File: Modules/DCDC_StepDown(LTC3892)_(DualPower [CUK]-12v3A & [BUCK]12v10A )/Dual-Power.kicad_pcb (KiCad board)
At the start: 4 copper layers, 58.4 x 55.9 mm, 81 parts, among them J1 Conn_02x05_Top_Bottom, J2 Conn_02x05_Top_Bottom, J3 Conn_01x02, Q1 BSC028N06LS3, Q2 BSC028N06LS3, Q3 BSC028N06LS3, Q4 BSC028N06LS3, Q5 BSC028N06LS3, U1 LTC3892EUHPBF, U2 LT1797

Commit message: update Dual-power
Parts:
- C11: value 1nF -> 6.8nF
- C12: value 100pF -> 47pF
- C21, C25: value 1nF -> 220pF
- C5: value 10nF -> 6.8nF
- C6: value 330pF -> 47pF
- R3: value 7.5K -> 10K
- R4: value 34.8K -> 10K
- R5: value 100K -> 31.6K

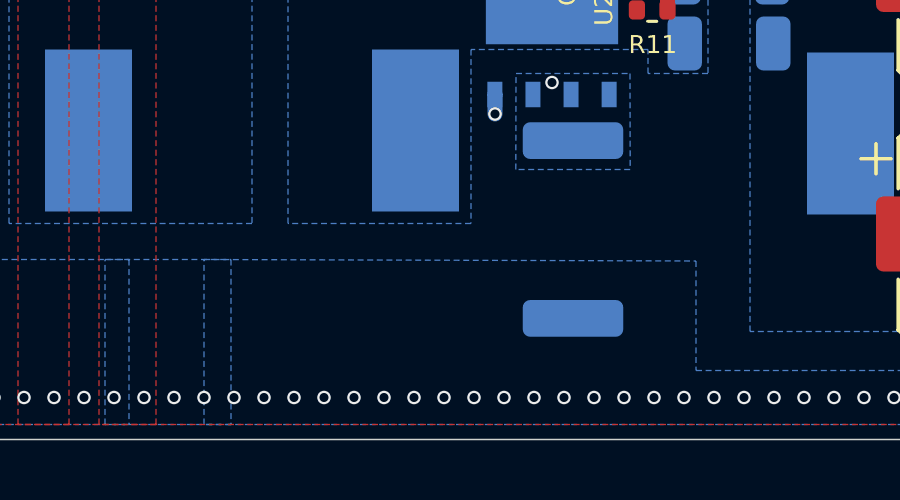
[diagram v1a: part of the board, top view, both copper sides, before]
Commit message: update dual_power
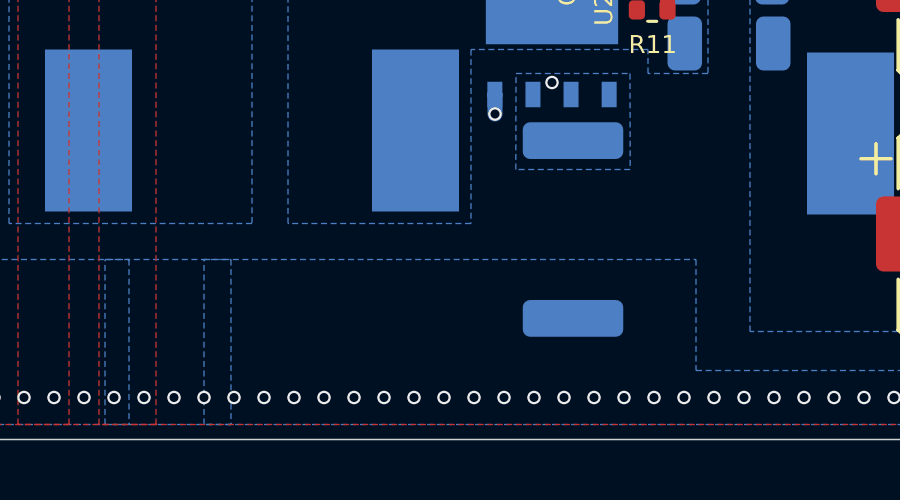
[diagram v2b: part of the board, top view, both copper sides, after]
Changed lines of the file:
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@@
     )
     (fp_poly (pts
+        (xy -1.675 0.1)
+        (xy -1.675 1.675)
+        (xy -0.1 1.675)
+        (xy -0.1 0.1)
+      ) (layer "F.Paste") (width 0.0254) (fill solid))
+    (fp_poly (pts
         (xy 0.1 0.1)
         (xy 0.1 1.675)
@@
         (xy -0.1 -1.675)
       ) (layer "F.Paste") (width 0.0254) (fill solid))
-    (fp_poly (pts
-        (xy -1.675 0.1)
-        (xy -1.675 1.675)
-        (xy -0.1 1.675)
-        (xy -0.1 0.1)
-      ) (layer "F.Paste") (width 0.0254) (fill solid))
-    (fp_line (start 2.667 -2.2352) (end 2.667 -2.667) (layer "F.SilkS") (width 0.1524))
     (fp_line (start -2.2352 -2.667) (end -2.667 -2.667) (layer "F.SilkS") (width 0.1524))
+    (fp_line (start 2.667 2.667) (end 2.667 2.2352) (layer "F.SilkS") (width 0.1524))
     (fp_line (start -2.667 -2.667) (end -2.667 -2.2352) (layer "F.SilkS") (width 0.1524))
+    (fp_line (start 2.667 -2.667) (end 2.2352 -2.667) (layer "F.SilkS") (width 0.1524))
+    (fp_line (start 2.2352 2.667) (end 2.667 2.667) (layer "F.SilkS") (width 0.1524))
+    (fp_line (start 2.667 -2.2352) (end 2.667 -2.667) (layer "F.SilkS") (width 0.1524))
     (fp_line (start -2.667 2.2352) (end -2.667 2.667) (layer "F.SilkS") (width 0.1524))
     (fp_line (start -2.667 2.667) (end -2.2352 2.667) (layer "F.SilkS") (width 0.1524))
-    (fp_line (start 2.2352 2.667) (end 2.667 2.667) (layer "F.SilkS") (width 0.1524))
-    (fp_line (start 2.667 -2.667) (end 2.2352 -2.667) (layer "F.SilkS") (width 0.1524))
-    (fp_line (start 2.667 2.667) (end 2.667 2.2352) (layer "F.SilkS") (width 0.1524))
-    (fp_line (start 0.889 -2.54) (end 0.6096 -2.54) (layer "F.Fab") (width 0.1524))
-    (fp_line (start -0.4064 2.54) (end -0.1016 2.54) (layer "F.Fab") (width 0.1524))
-    (fp_line (start 1.0922 2.54) (end 1.397 2.54) (layer "F.Fab") (width 0.1524))
-    (fp_line (start 0.4064 -2.54) (end 0.1016 -2.54) (layer "F.Fab") (width 0.1524))
-    (fp_line (start -1.6002 -2.54) (end -1.905 -2.54) (layer "F.Fab") (width 0.1524))
-    (fp_line (start 2.54 0.889) (end 2.54 0.6096) (layer "F.Fab") (width 0.1524))
-    (fp_line (start 2.54 -0.1016) (end 2.54 -0.4064) (layer "F.Fab") (width 0.1524))
     (fp_line (start 2.54 -0.6096) (end 2.54 -0.889) (layer "F.Fab") (width 0.1524))
-    (fp_line (start -2.54 -1.27) (end -1.27 -2.54) (layer "F.Fab") (width 0.1524))
-    (fp_line (start -2.54 2.54) (end 2.54 2.54) (layer "F.Fab") (width 0.1524))
-    (fp_line (start -2.54 -0.889) (end -2.54 -0.6096) (layer "F.Fab") (width 0.1524))
-    (fp_line (start -1.905 2.54) (end -1.6002 2.54) (layer "F.Fab") (width 0.1524))
+    (fp_line (start -0.1016 -2.54) (end -0.4064 -2.54) (layer "F.Fab") (width 0.1524))
+    (fp_line (start 0.4064 -2.54) (end 0.1016 -2.54) (layer "F.Fab") (width 0.1524))
     (fp_line (start -0.6096 -2.54) (end -0.889 -2.54) (layer "F.Fab") (width 0.1524))
+    (fp_line (start -2.54 -1.27) (end -1.27 -2.54) (layer "F.Fab") (width 0.1524))
+    (fp_line (start 2.54 -2.54) (end -2.54 -2.54) (layer "F.Fab") (width 0.1524))
     (fp_line (start 2.54 0.4064) (end 2.54 0.1016) (layer "F.Fab") (width 0.1524))
-    (fp_line (start 2.54 1.905) (end 2.54 1.6002) (layer "F.Fab") (width 0.1524))
-    (fp_line (start -2.54 -0.4064) (end -2.54 -0.1016) (layer "F.Fab") (width 0.1524))
     (fp_line (start -2.54 -2.54) (end -2.54 2.54) (layer "F.Fab") (width 0.1524))
-    (fp_line (start 2.54 -1.0922) (end 2.54 -1.397) (layer "F.Fab") (width 0.1524))
-    (fp_line (start -0.1016 -2.54) (end -0.4064 -2.54) (layer "F.Fab") (width 0.1524))
-    (fp_line (start 2.54 -2.54) (end -2.54 -2.54) (layer "F.Fab") (width 0.1524))
-    (fp_line (start -0.889 2.54) (end -0.6096 2.54) (layer "F.Fab") (width 0.1524))
+    (fp_line (start 0.1016 2.54) (end 0.4064 2.54) (layer "F.Fab") (width 0.1524))
+    (fp_line (start 2.54 1.397) (end 2.54 1.0922) (layer "F.Fab") (width 0.1524))
     (fp_line (start -2.54 1.0922) (end -2.54 1.397) (layer "F.Fab") (width 0.1524))
+    (fp_line (start -1.905 2.54) (end -1.6002 2.54) (layer "F.Fab") (width 0.1524))
+    (fp_line (start -2.54 -0.889) (end -2.54 -0.6096) (layer "F.Fab") (width 0.1524))
+    (fp_line (start 1.397 -2.54) (end 1.0922 -2.54) (layer "F.Fab") (width 0.1524))
+    (fp_line (start -2.54 -0.4064) (end -2.54 -0.1016) (layer "F.Fab") (width 0.1524))
+    (fp_line (start 2.54 2.54) (end 2.54 -2.54) (layer "F.Fab") (width 0.1524))
     (fp_line (start 2.54 -1.6002) (end 2.54 -1.905) (layer "F.Fab") (width 0.1524))
+    (fp_line (start -2.54 1.6002) (end -2.54 1.905) (layer "F.Fab") (width 0.1524))
+    (fp_line (start -2.54 -1.397) (end -2.54 -1.0922) (layer "F.Fab") (width 0.1524))
+    (fp_line (start -1.0922 -2.54) (end -1.397 -2.54) (layer "F.Fab") (width 0.1524))
+    (fp_line (start 2.54 0.889) (end 2.54 0.6096) (layer "F.Fab") (width 0.1524))
+    (fp_line (start 2.54 -0.1016) (end 2.54 -0.4064) (layer "F.Fab") (width 0.1524))
+    (fp_line (start -0.889 2.54) (end -0.6096 2.54) (layer "F.Fab") (width 0.1524))
+    (fp_line (start 2.54 1.905) (end 2.54 1.6002) (layer "F.Fab") (width 0.1524))
     (fp_line (start -2.54 0.6096) (end -2.54 0.889) (layer "F.Fab") (width 0.1524))
-    (fp_line (start -2.54 -1.905) (end -2.54 -1.6002) (layer "F.Fab") (width 0.1524))
-    (fp_line (start -1.397 2.54) (end -1.0922 2.54) (layer "F.Fab") (width 0.1524))
     (fp_line (start 1.6002 2.54) (end 1.905 2.54) (layer "F.Fab") (width 0.1524))
+    (fp_line (start -2.54 2.54) (end 2.54 2.54) (layer "F.Fab") (width 0.1524))
+    (fp_line (start -1.6002 -2.54) (end -1.905 -2.54) (layer "F.Fab") (width 0.1524))
+    (fp_line (start 1.0922 2.54) (end 1.397 2.54) (layer "F.Fab") (width 0.1524))
+    (fp_line (start 0.889 -2.54) (end 0.6096 -2.54) (layer "F.Fab") (width 0.1524))
+    (fp_line (start 2.54 -1.0922) (end 2.54 -1.397) (layer "F.Fab") (width 0.1524))
+    (fp_line (start -0.4064 2.54) (end -0.1016 2.54) (layer "F.Fab") (width 0.1524))
     (fp_line (start -2.54 0.1016) (end -2.54 0.4064) (layer "F.Fab") (width 0.1524))
-    (fp_line (start 2.54 2.54) (end 2.54 -2.54) (layer "F.Fab") (width 0.1524))
-    (fp_line (start -2.54 1.6002) (end -2.54 1.905) (layer "F.Fab") (width 0.1524))
-    (fp_line (start -2.54 -1.397) (end -2.54 -1.0922) (layer "F.Fab") (width 0.1524))
-    (fp_line (start 0.6096 2.54) (end 0.889 2.54) (layer "F.Fab") (width 0.1524))
-    (fp_line (start 0.1016 2.54) (end 0.4064 2.54) (layer "F.Fab") (width 0.1524))
-    (fp_line (start 1.397 -2.54) (end 1.0922 -2.54) (layer "F.Fab") (width 0.1524))
+    (fp_line (start -1.397 2.54) (end -1.0922 2.54) (layer "F.Fab") (width 0.1524))
     (fp_line (start 1.905 -2.54) (end 1.6002 -2.54) (layer "F.Fab") (width 0.1524))
-    (fp_line (start 2.54 1.397) (end 2.54 1.0922) (layer "F.Fab") (width 0.1524))
-    (fp_line (start -1.0922 -2.54) (end -1.397 -2.54) (layer "F.Fab") (width 0.1524))
+    (fp_line (start 0.6096 2.54) (end 0.889 2.54) (layer "F.Fab") (width 0.1524))
+    (fp_line (start -2.54 -1.905) (end -2.54 -1.6002) (layer "F.Fab") (width 0.1524))
     (pad "1" smd rect locked (at -2.4524 -1.75) (size 0.8048 0.3) (layers "F.Cu" "F.Paste" "F.Mask")
       (net 27 "Net-(R5-Pad1)") (pinfunction "FREQ") (pintype "passive"))
@@
         (xy -1.06 -0.414)
       ) (layer "B.Paste") (width 0.01) (fill solid))
-    (fp_line (start 1.985 2.685) (end 1.985 -2.685) (layer "B.SilkS") (width 0.127))
     (fp_line (start -1.985 -2.685) (end -1.985 2.685) (layer "B.SilkS") (width 0.127))
+    (fp_line (start 1.985 2.685) (end 1.985 -2.685) (layer "B.SilkS") (width 0.127))
     (fp_circle (center -0.9 -4.1) (end -0.8 -4.1) (layer "B.SilkS") (width 0.2) (fill none))
-    (fp_line (start -2.235 3.81) (end 2.235 3.81) (layer "B.CrtYd") (width 0.05))
     (fp_line (start 2.235 3.81) (end 2.235 -3.81) (layer "B.CrtYd") (width 0.05))
+    (fp_line (start -2.235 3.81) (end 2.235 3.81) (layer "B.CrtYd") (width 0.05))
     (fp_line (start -2.235 -3.81) (end -2.235 3.81) (layer "B.CrtYd") (width 0.05))
     (fp_line (start 2.235 -3.81) (end -2.235 -3.81) (layer "B.CrtYd") (width 0.05))
+    (fp_line (start -1.985 -2.685) (end -1.985 2.685) (layer "B.Fab") (width 0.127))
+    (fp_line (start 1.985 -2.685) (end -1.985 -2.685) (layer "B.Fab") (width 0.127))
     (fp_line (start 1.985 2.685) (end 1.985 -2.685) (layer "B.Fab") (width 0.127))
     (fp_line (start -1.985 2.685) (end 1.985 2.685) (layer "B.Fab") (width 0.127))
-    (fp_line (start 1.985 -2.685) (end -1.985 -2.685) (layer "B.Fab") (width 0.127))
-    (fp_line (start -1.985 -2.685) (end -1.985 2.685) (layer "B.Fab") (width 0.127))
     (fp_circle (center -0.9 -4.1) (end -0.8 -4.1) (layer "B.Fab") (width 0.2) (fill none))
     (pad "1" smd rect locked (at -0.92 -2.856 180) (size 1.39 1.4) (layers "B.Cu" "B.Paste" "B.Mask")
@@
         (xy 126.4 114.7)
         (xy 126.4 109.2)
-        (xy 142.8 109.25)
+        (xy 142.8 109.2)
         (xy 142.8 112.9)
         (xy 165.6 112.899674)
